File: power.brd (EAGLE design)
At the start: 136 x 136 mm, 31 parts, among them CN1 21700, CN2 21700, CN3 1 X 3 HEADER, CN4 21700, Q6 IRLML6244, Q7 IRLML6244, U17 MAX17320G20+

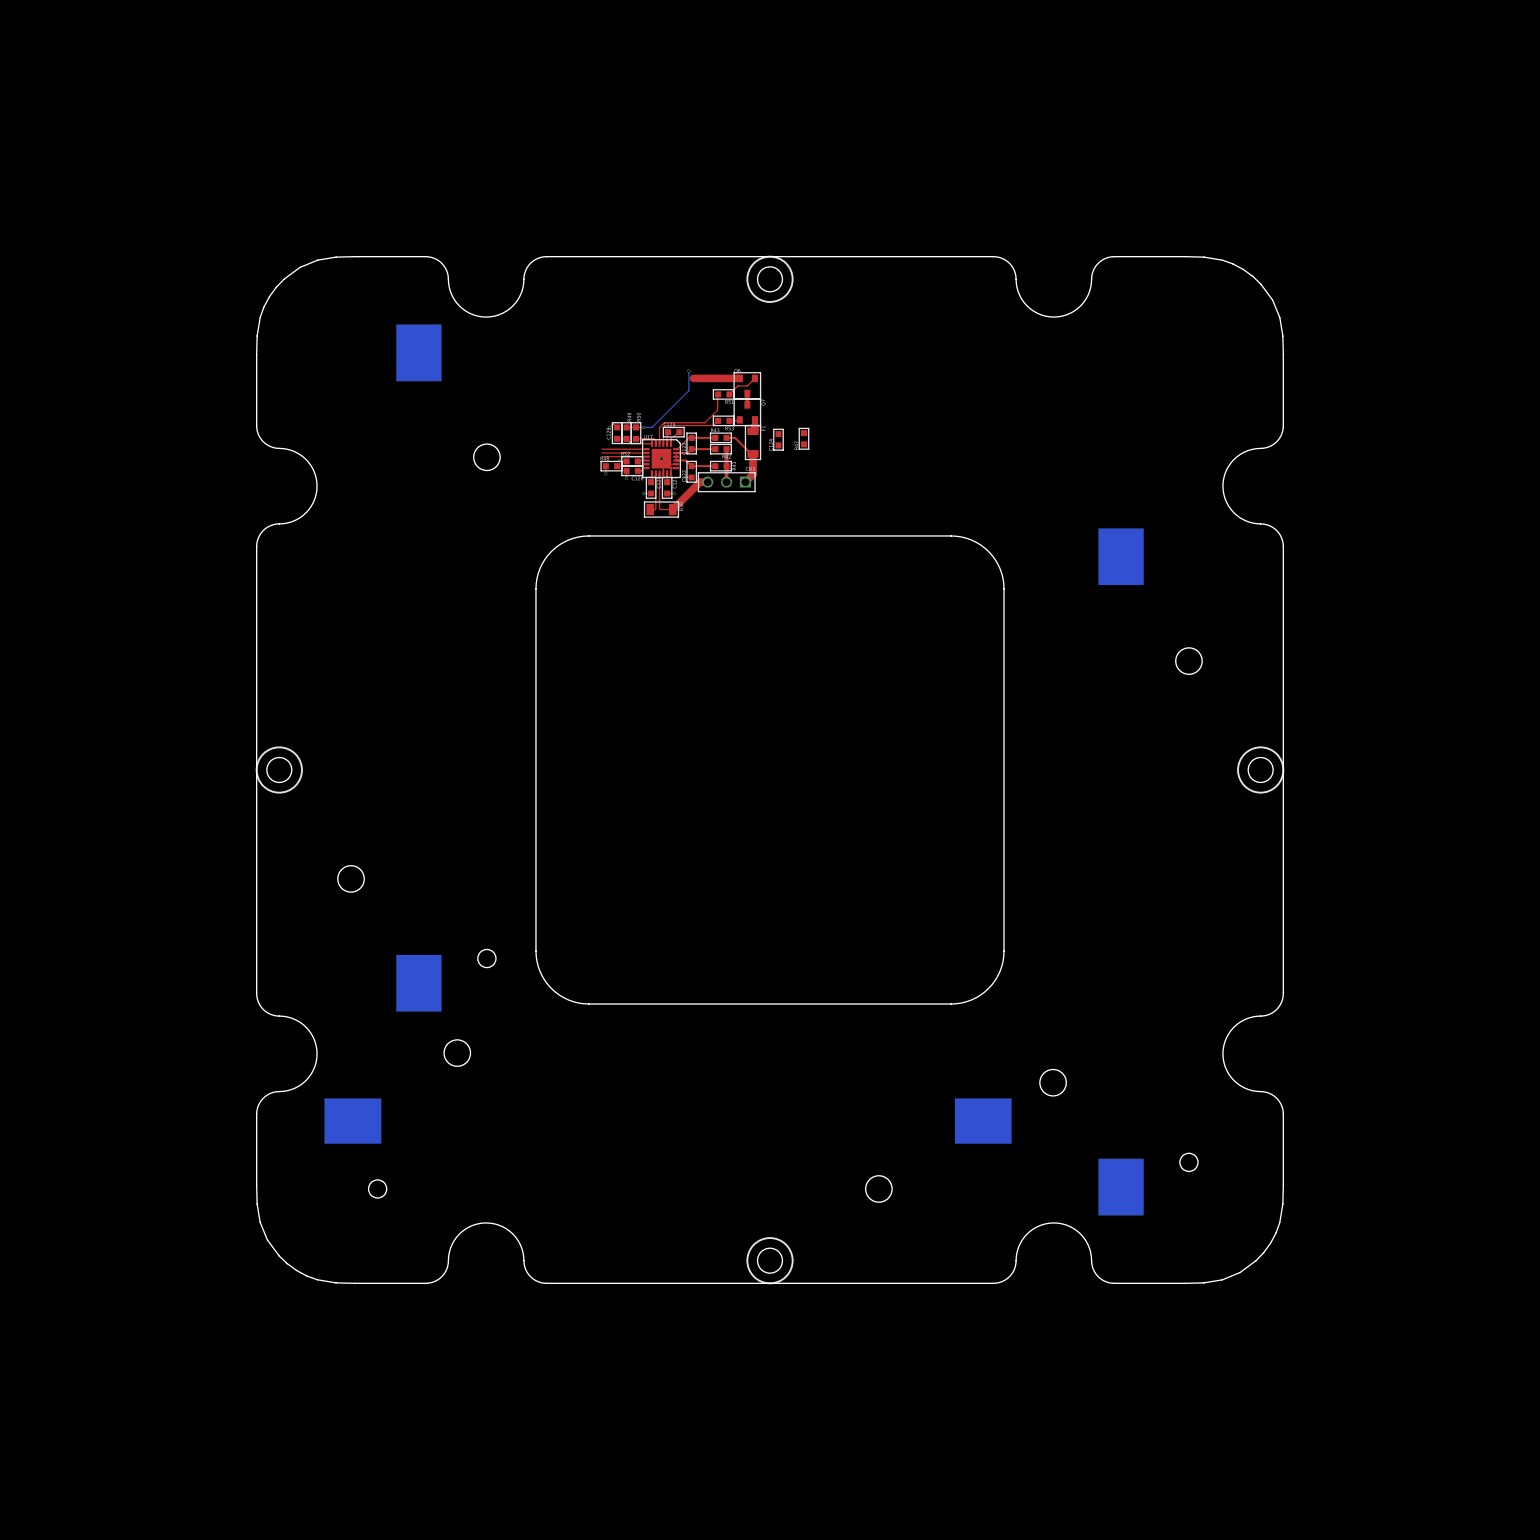
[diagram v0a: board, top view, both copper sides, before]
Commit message: New more simple desing
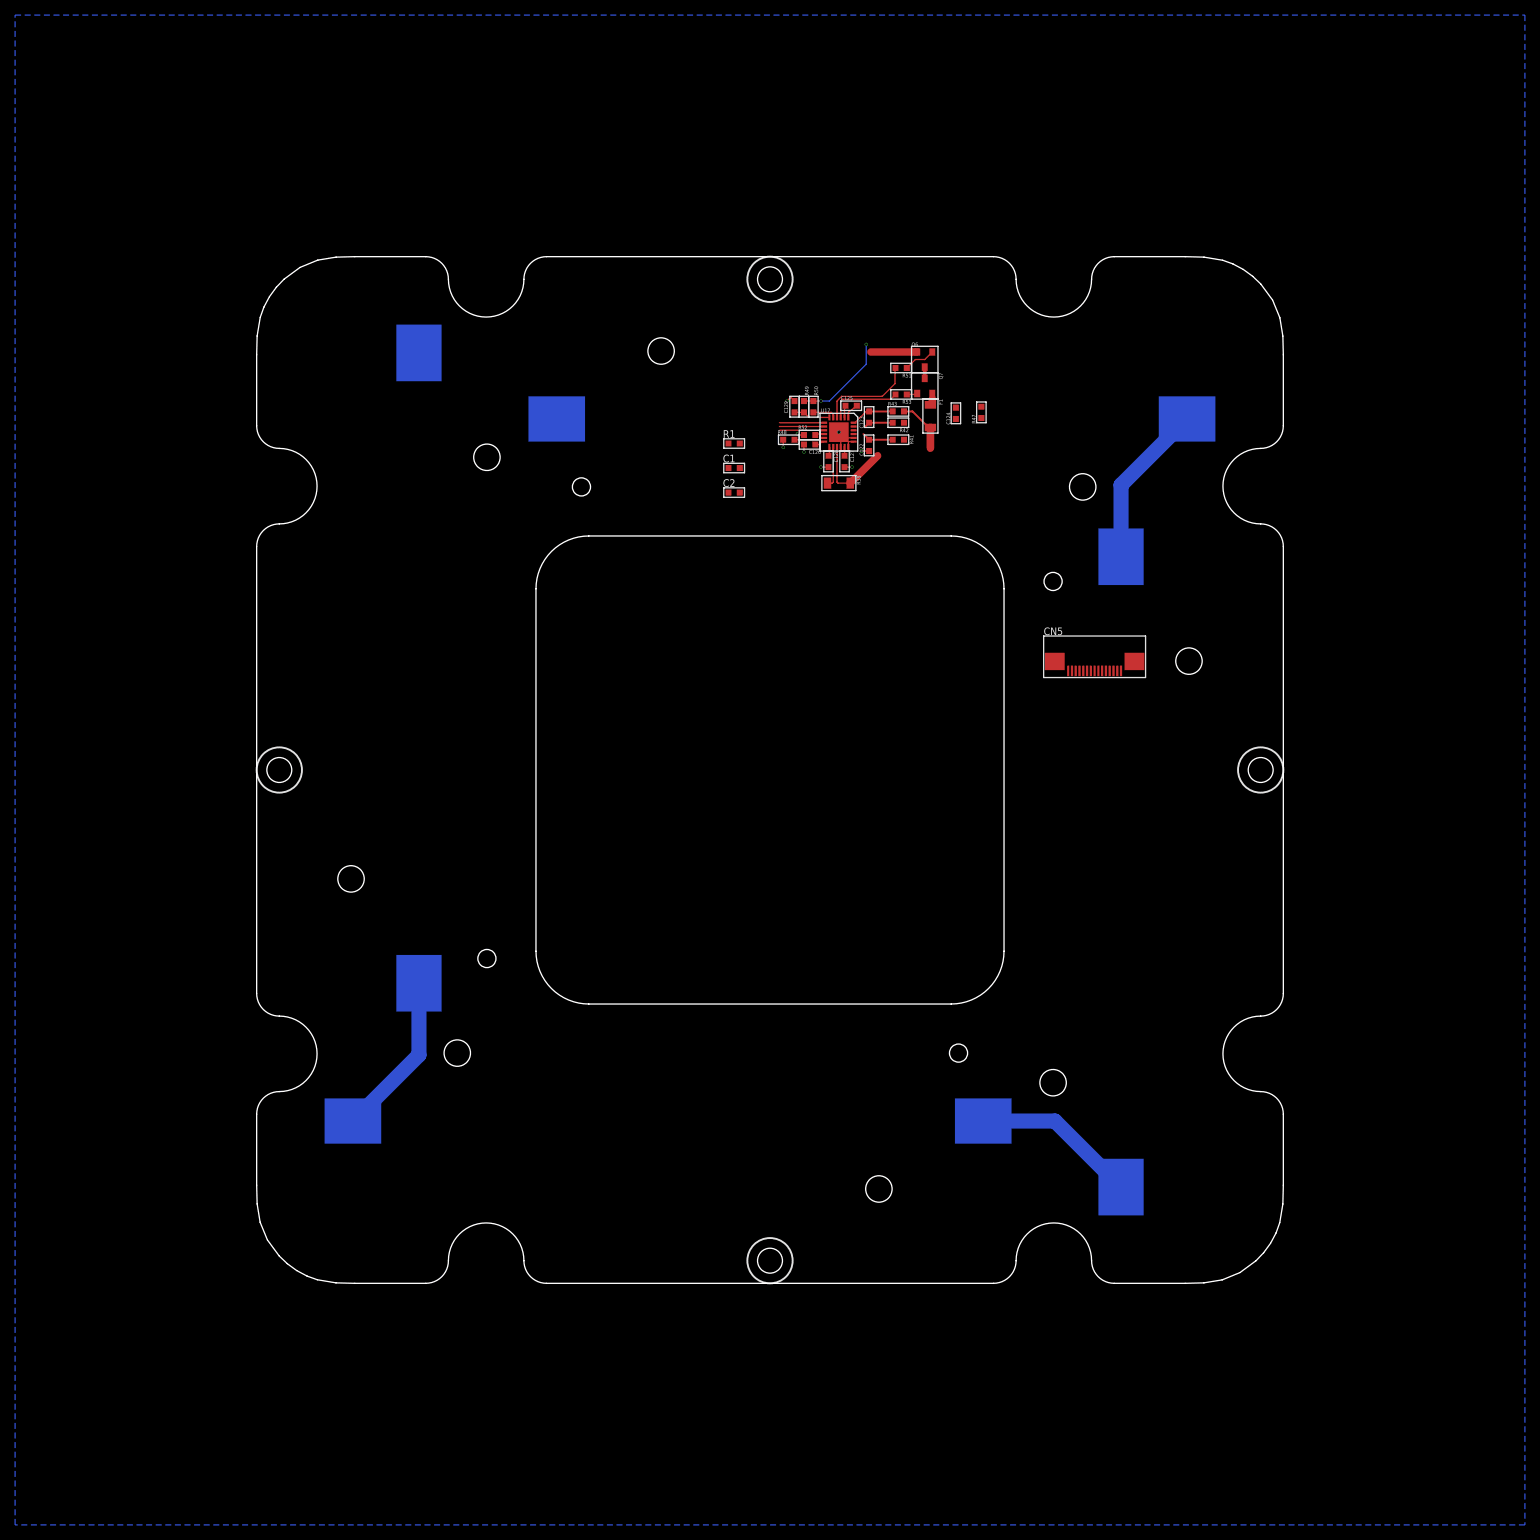
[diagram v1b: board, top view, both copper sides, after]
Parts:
- added C1, C2: 100nF 16V, CAPACITORS:0603
- added CN5: 15PIN 0.5MM, CONNECTORs:SFV15R-1STE1HLF
- added R1: 47R, r_0603:0603
- CN3: value 1 X 3 HEADER -> 21700; device CONNECTORs:3PIN_HEADER -> CONNECTORs:1122
- moved CN3 85.0 mm to (-13.5, -46.5), flipped to the bottom, turned to 180 degrees
- moved CN1 68.5 mm to (13.5, 46.5), turned to 0 degrees
- moved CN2 68.5 mm to (46.5, -13.5), turned to 90 degrees
- moved C122 23.8 mm to (13.1, 43.0)
- moved C123 23.8 mm to (13.1, 46.8)
- moved C124 23.8 mm to (24.6, 47.2)
- moved C125 23.8 mm to (10.8, 48.2)
- moved C126 23.8 mm to (5.25, 43.1)
- moved C127 23.8 mm to (9.88, 40.9)
- moved C128 23.8 mm to (7.75, 40.9)
- moved C129 23.8 mm to (3.25, 48.1)
- moved F1 23.8 mm to (21.2, 46.9)
- moved Q6 23.8 mm to (20.5, 54.4)
- moved Q7 23.8 mm to (20.5, 50.9)
- moved R38 23.8 mm to (9.12, 38.0)
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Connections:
- removed net N$40: C122.2, C123.1, R41.2, R42.2, U17.21, U17.22, U17.23
- new net N$1: C1.1, C122.2, R41.2, U17.21
- new net N$2: C123.1, C2.2, R42.2, U17.23
- new net N$3: C1.2, C2.1, R1.2, U17.22
- new net N$4: CN1.-, CN2.+, R42.1
- new net N$5: CN2.-, CN3.+, R1.1
- net N$36: now also CN1.+; no longer CN3.1
- net PACK_MID: now also CN3.-, CN4.+; no longer CN3.2, R42.1
- net PGND: now also CN4.-; no longer CN3.3
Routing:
- net N$5: track 0.00 -> 21.9 mm
- net N$4: track 0.00 -> 21.9 mm
- net PACK_MID: track 4.38 -> 21.9 mm
- net N$40: track 11.9 -> 0.00 mm
- net N$1: track 0.00 -> 4.19 mm
- net N$2: track 0.00 -> 3.83 mm
- net N$36: track 8.54 -> 7.13 mm
- net PGND: track 23.6 -> 22.6 mm
- added copper zone on layer 16, net PGND
